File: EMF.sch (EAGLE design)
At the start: 23 parts, among them X1 22-23-2021

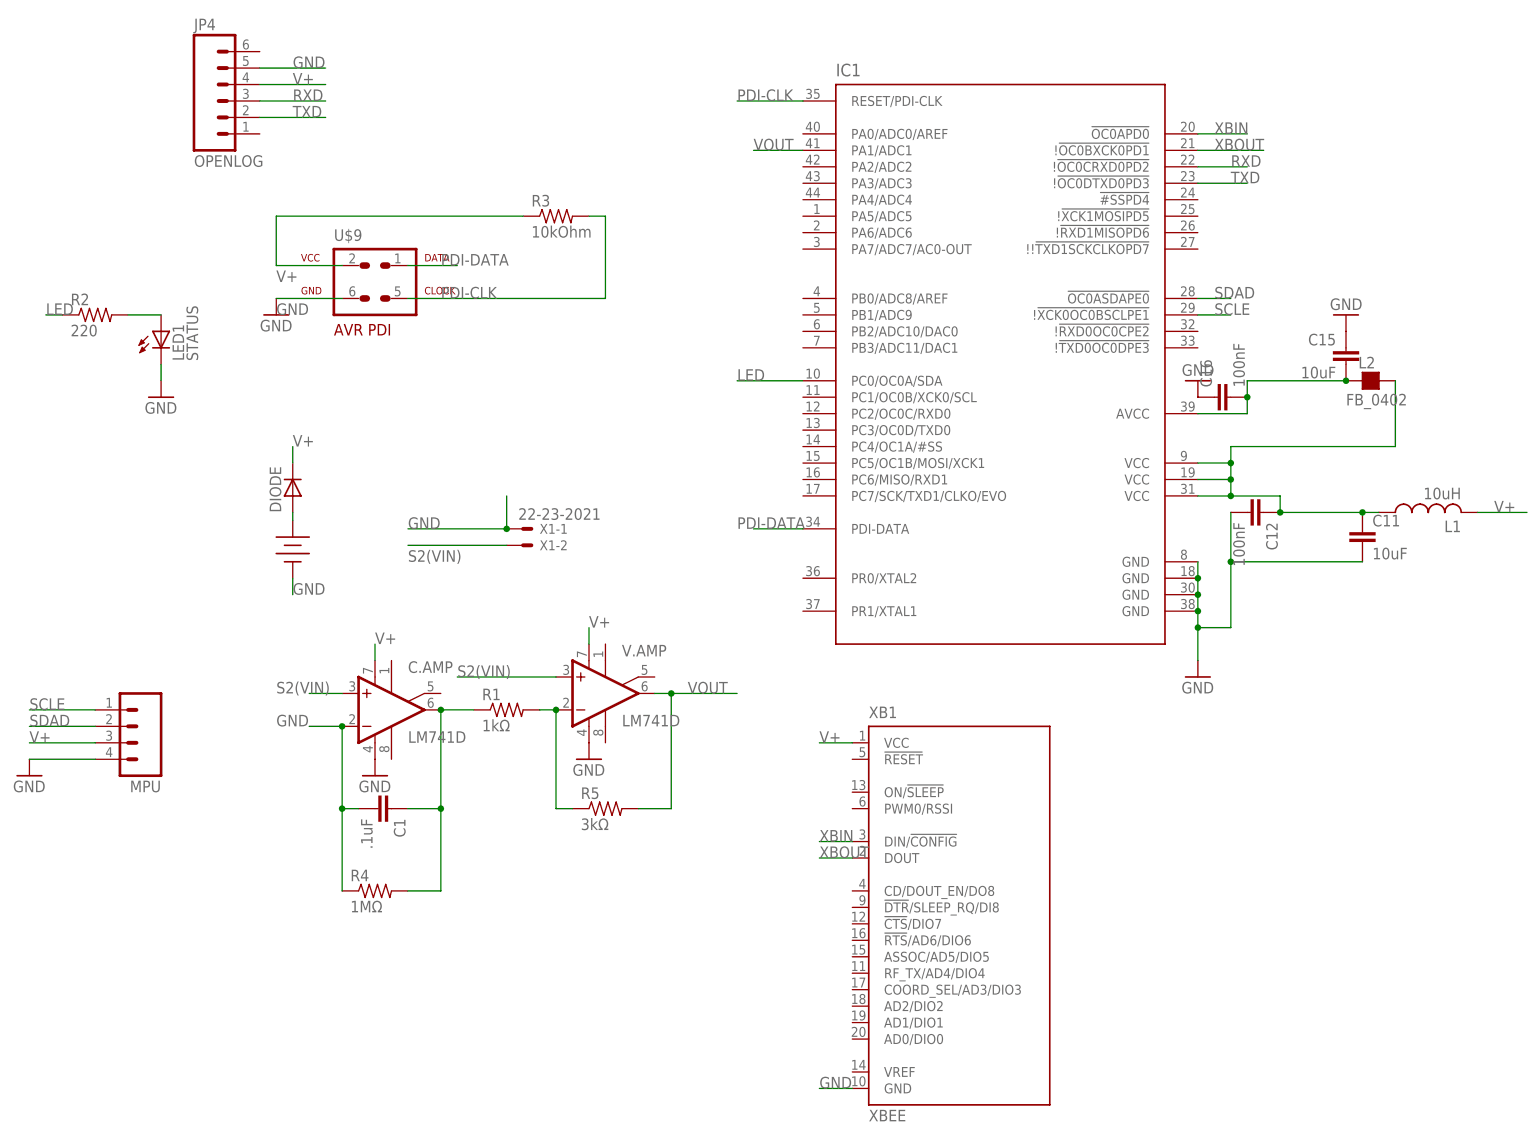
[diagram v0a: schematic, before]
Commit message: fixing stuff
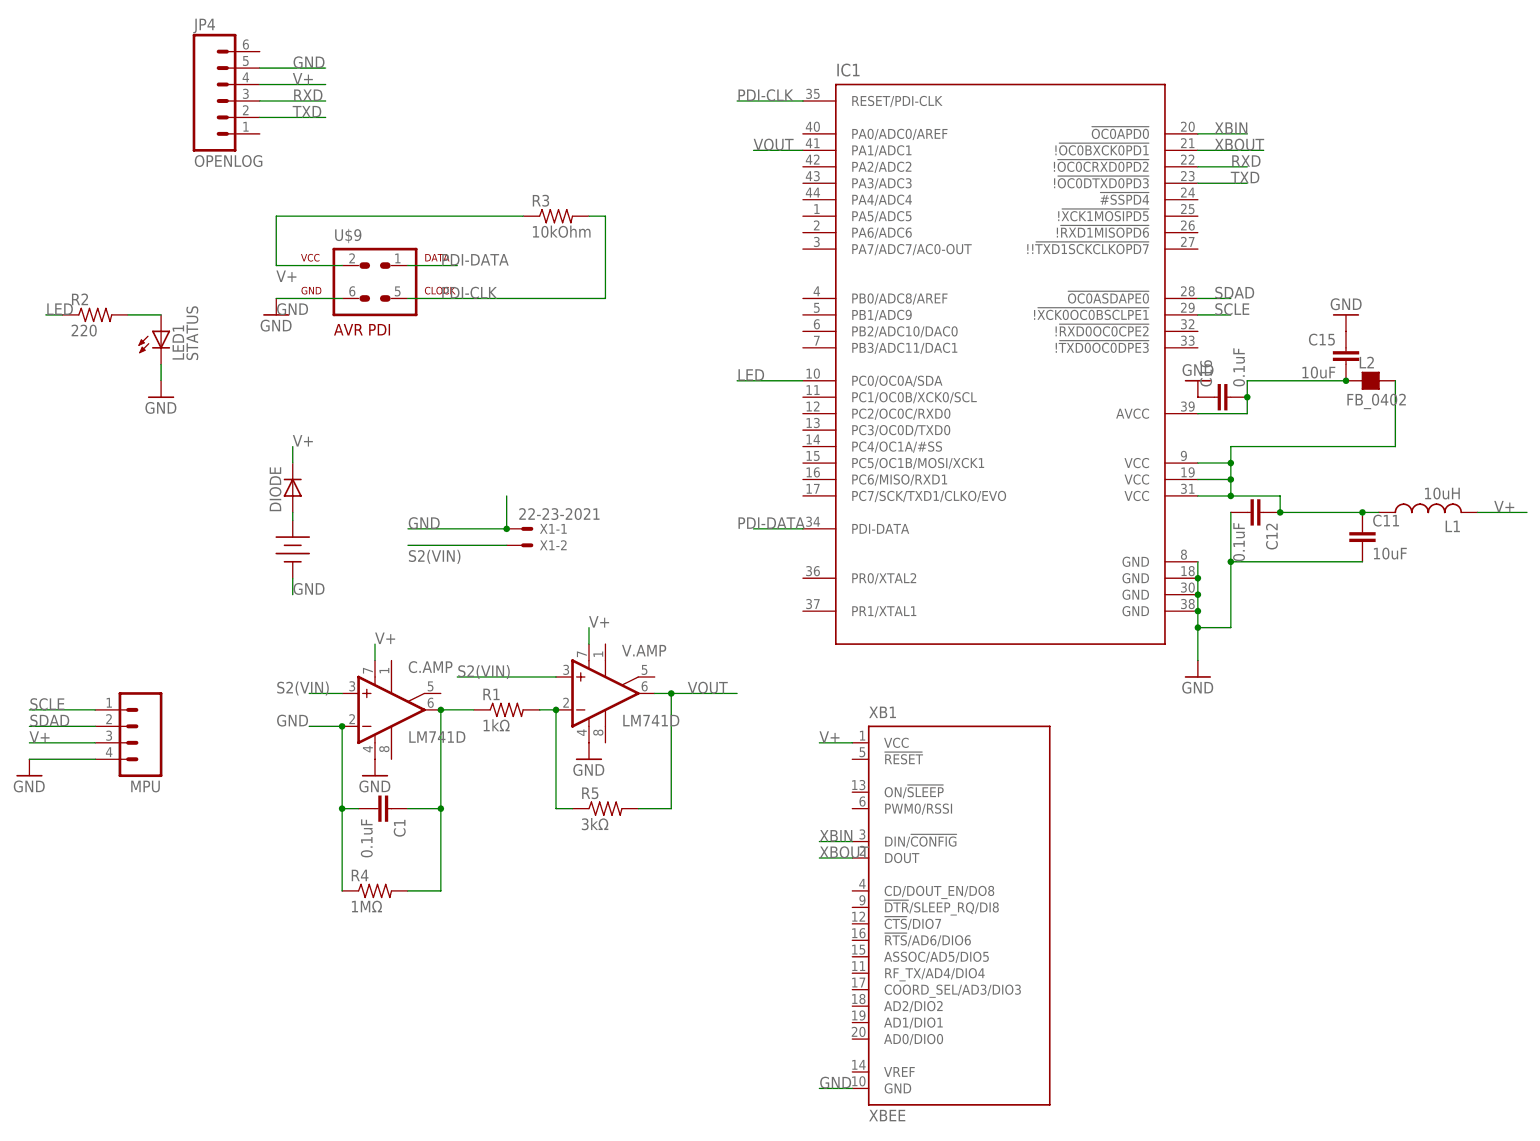
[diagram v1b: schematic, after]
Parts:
- C1: value .1uF -> 0.1uF
- C12, C16: value 100nF -> 0.1uF
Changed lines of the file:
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@@
 <grid distance="0.1" unitdist="inch" unit="inch" style="lines" multiple="1" display="no" altdistance="0.01" altunitdist="inch" altunit="inch"/>
 <layers>
-<layer number="1" name="Top" color="4" fill="1" visible="no" active="no"/>
-<layer number="2" name="Route2" color="1" fill="3" visible="no" active="no"/>
-<layer number="3" name="Route3" color="4" fill="3" visible="no" active="no"/>
-<layer number="4" name="Route4" color="1" fill="4" visible="no" active="no"/>
-<layer number="5" name="Route5" color="4" fill="4" visible="no" active="no"/>
-<layer number="6" name="Route6" color="1" fill="8" visible="no" active="no"/>
-<layer number="7" name="Route7" color="4" fill="8" visible="no" active="no"/>
-<layer number="8" name="Route8" color="1" fill="2" visible="no" active="no"/>
-<layer number="9" name="Route9" color="4" fill="2" visible="no" active="no"/>
-<layer number="10" name="Route10" color="1" fill="7" visible="no" active="no"/>
-<layer number="11" name="Route11" color="4" fill="7" visible="no" active="no"/>
-<layer number="12" name="Route12" color="1" fill="5" visible="no" active="no"/>
-<layer number="13" name="Route13" color="4" fill="5" visible="no" active="no"/>
-<layer number="14" name="Route14" color="1" fill="6" visible="no" active="no"/>
-<layer number="15" name="Route15" color="4" fill="6" visible="no" active="no"/>
-<layer number="16" name="Bottom" color="1" fill="1" visible="no" active="no"/>
-<layer number="17" name="Pads" color="2" fill="1" visible="no" active="no"/>
-<layer number="18" name="Vias" color="2" fill="1" visible="no" active="no"/>
-<layer number="19" name="Unrouted" color="6" fill="1" visible="no" active="no"/>
-<layer number="20" name="Dimension" color="24" fill="1" visible="no" active="no"/>
-<layer number="21" name="tPlace" color="7" fill="1" visible="no" active="no"/>
-<layer number="22" name="bPlace" color="7" fill="1" visible="no" active="no"/>
-<layer number="23" name="tOrigins" color="15" fill="1" visible="no" active="no"/>
-<layer number="24" name="bOrigins" color="15" fill="1" visible="no" active="no"/>
-<layer number="25" name="tNames" color="7" fill="1" visible="no" active="no"/>
-<layer number="26" name="bNames" color="7" fill="1" visible="no" active="no"/>
-<layer number="27" name="tValues" color="7" fill="1" visible="no" active="no"/>
-<layer number="28" name="bValues" color="7" fill="1" visible="no" active="no"/>
+<layer number="1" name="Top" color="4" fill="1" visible="yes" active="no"/>
+<layer number="2" name="Route2" color="1" fill="3" visible="yes" active="no"/>
+<layer number="3" name="Route3" color="4" fill="3" visible="yes" active="no"/>
+<layer number="4" name="Route4" color="1" fill="4" visible="yes" active="no"/>
+<layer number="5" name="Route5" color="4" fill="4" visible="yes" active="no"/>
+<layer number="6" name="Route6" color="1" fill="8" visible="yes" active="no"/>
+<layer number="7" name="Route7" color="4" fill="8" visible="yes" active="no"/>
+<layer number="8" name="Route8" color="1" fill="2" visible="yes" active="no"/>
+<layer number="9" name="Route9" color="4" fill="2" visible="yes" active="no"/>
+<layer number="10" name="Route10" color="1" fill="7" visible="yes" active="no"/>
+<layer number="11" name="Route11" color="4" fill="7" visible="yes" active="no"/>
+<layer number="12" name="Route12" color="1" fill="5" visible="yes" active="no"/>
+<layer number="13" name="Route13" color="4" fill="5" visible="yes" active="no"/>
+<layer number="14" name="Route14" color="1" fill="6" visible="yes" active="no"/>
+<layer number="15" name="Route15" color="4" fill="6" visible="yes" active="no"/>
+<layer number="16" name="Bottom" color="1" fill="1" visible="yes" active="no"/>
+<layer number="17" name="Pads" color="2" fill="1" visible="yes" active="no"/>
+<layer number="18" name="Vias" color="2" fill="1" visible="yes" active="no"/>
+<layer number="19" name="Unrouted" color="6" fill="1" visible="yes" active="no"/>
+<layer number="20" name="Dimension" color="24" fill="1" visible="yes" active="no"/>
+<layer number="21" name="tPlace" color="7" fill="1" visible="yes" active="no"/>
+<layer number="22" name="bPlace" color="7" fill="1" visible="yes" active="no"/>
+<layer number="23" name="tOrigins" color="15" fill="1" visible="yes" active="no"/>
+<layer number="24" name="bOrigins" color="15" fill="1" visible="yes" active="no"/>
+<layer number="25" name="tNames" color="7" fill="1" visible="yes" active="no"/>
+<layer number="26" name="bNames" color="7" fill="1" visible="yes" active="no"/>
+<layer number="27" name="tValues" color="7" fill="1" visible="yes" active="no"/>
+<layer number="28" name="bValues" color="7" fill="1" visible="yes" active="no"/>
 <layer number="29" name="tStop" color="7" fill="3" visible="no" active="no"/>
 <layer number="30" name="bStop" color="7" fill="6" visible="no" active="no"/>
@@
 <layer number="35" name="tGlue" color="7" fill="4" visible="no" active="no"/>
 <layer number="36" name="bGlue" color="7" fill="5" visible="no" active="no"/>
-<layer number="37" name="tTest" color="7" fill="1" visible="no" active="no"/>
-<layer number="38" name="bTest" color="7" fill="1" visible="no" active="no"/>
+<layer number="37" name="tTest" color="7" fill="1" visible="yes" active="no"/>
+<layer number="38" name="bTest" color="7" fill="1" visible="yes" active="no"/>
 <layer number="39" name="tKeepout" color="4" fill="11" visible="no" active="no"/>
 <layer number="40" name="bKeepout" color="1" fill="11" visible="no" active="no"/>
@@
 <layer number="44" name="Drills" color="7" fill="1" visible="no" active="no"/>
 <layer number="45" name="Holes" color="7" fill="1" visible="no" active="no"/>
-<layer number="46" name="Milling" color="3" fill="1" visible="no" active="no"/>
-<layer number="47" name="Measures" color="7" fill="1" visible="no" active="no"/>
-<layer number="48" name="Document" color="7" fill="1" visible="no" active="no"/>
-<layer number="49" name="Reference" color="7" fill="1" visible="no" active="no"/>
-<layer number="50" name="dxf" color="7" fill="1" visible="no" active="no"/>
-<layer number="51" name="tDocu" color="7" fill="1" visible="no" active="no"/>
-<layer number="52" name="bDocu" color="7" fill="1" visible="no" active="no"/>
-<layer number="53" name="tGND_GNDA" color="7" fill="1" visible="no" active="no"/>
-<layer number="54" name="bGND_GNDA" color="7" fill="1" visible="no" active="no"/>
-<layer number="56" name="wert" color="7" fill="1" visible="no" active="no"/>
-<layer number="60" name="p_dimension" color="7" fill="1" visible="no" active="no"/>
-<layer number="61" name="pt_docu" color="7" fill="1" visible="no" active="no"/>
+<layer number="46" name="Milling" color="3" fill="1" visible="yes" active="no"/>
+<layer number="47" name="Measures" color="7" fill="1" visible="yes" active="no"/>
+<layer number="48" name="Document" color="7" fill="1" visible="yes" active="no"/>
+<layer number="49" name="Reference" color="7" fill="1" visible="yes" active="no"/>
+<layer number="50" name="dxf" color="7" fill="1" visible="yes" active="no"/>
+<layer number="51" name="tDocu" color="7" fill="1" visible="yes" active="no"/>
+<layer number="52" name="bDocu" color="7" fill="1" visible="yes" active="no"/>
+<layer number="53" name="tGND_GNDA" color="7" fill="1" visible="yes" active="no"/>
+<layer number="54" name="bGND_GNDA" color="7" fill="1" visible="yes" active="no"/>
+<layer number="56" name="wert" color="7" fill="1" visible="yes" active="no"/>
+<layer number="60" name="p_dimension" color="7" fill="1" visible="yes" active="no"/>
+<layer number="61" name="pt_docu" color="7" fill="1" visible="yes" active="no"/>
 <layer number="88" name="SimResults" color="9" fill="1" visible="yes" active="yes"/>
 <layer number="89" name="SimProbes" color="9" fill="1" visible="yes" active="yes"/>
@@
 <part name="L2" library="rc-master-smd" deviceset="FB_" device="0402"/>
 <part name="C15" library="SparkFun" deviceset="CAP" device="0805" value="10uF"/>
-<part name="C16" library="SparkFun" deviceset="CAP" device="0805" value="100nF"/>
+<part name="C16" library="SparkFun" deviceset="CAP" device="0805" value="0.1uF"/>
 <part name="GND32" library="SparkFun-Aesthetics" deviceset="GND" device=""/>
 <part name="GND33" library="SparkFun-Aesthetics" deviceset="GND" device=""/>
-<part name="C12" library="SparkFun" deviceset="CAP" device="0805" value="100nF"/>
+<part name="C12" library="SparkFun" deviceset="CAP" device="0805" value="0.1uF"/>
 <part name="U$9" library="avr-7" deviceset="AVR-PDI" device="VERT"/>
 <part name="GND4" library="SparkFun-Aesthetics" deviceset="GND" device=""/>
@@
 <part name="R4" library="resistor" library_urn="urn:adsk.eagle:library:348" deviceset="R-US_" device="M2012" package3d_urn="urn:adsk.eagle:package:26082/1" value="1MΩ"/>
 <part name="R5" library="resistor" library_urn="urn:adsk.eagle:library:348" deviceset="R-US_" device="M2012" package3d_urn="urn:adsk.eagle:package:26082/1" value="3kΩ"/>
-<part name="C1" library="SparkFun" deviceset="CAP" device="0805" value=".1uF"/>
+<part name="C1" library="SparkFun" deviceset="CAP" device="0805" value="0.1uF"/>
 <part name="MPU" library="con-amp-quick" deviceset="M04" device=""/>
 <part name="GND20" library="SparkFun-Aesthetics" deviceset="GND" device=""/>
